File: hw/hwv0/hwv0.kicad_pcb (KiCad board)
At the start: 2 copper layers, 60.3 x 54.6 mm, 29 parts, among them J1 AVR-ISP-6, J2 PWR_IN_7-12V, J3 RS232, SW1 SW_Push, U1 ATtiny84A-MU, U2 LCD_1602, U3 MAX232I, U4 L7805

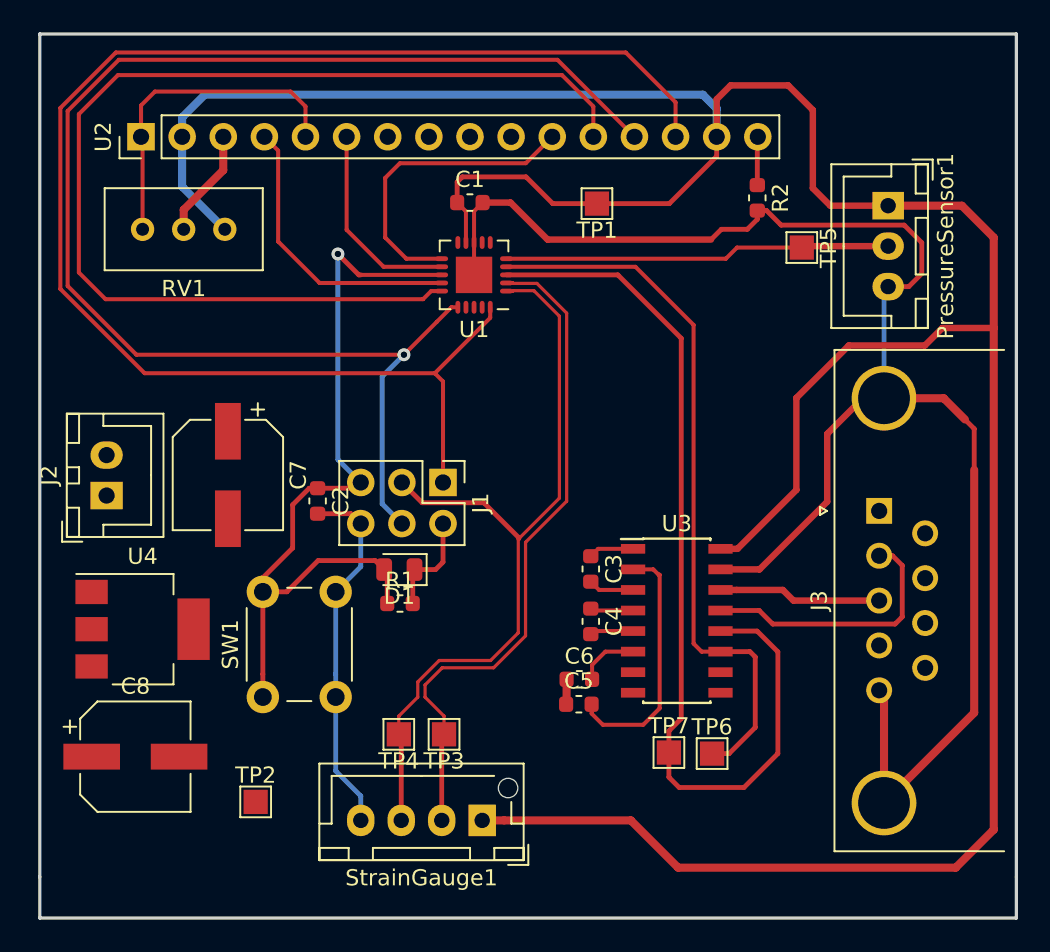
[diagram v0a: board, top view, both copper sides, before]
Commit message: finished PCB
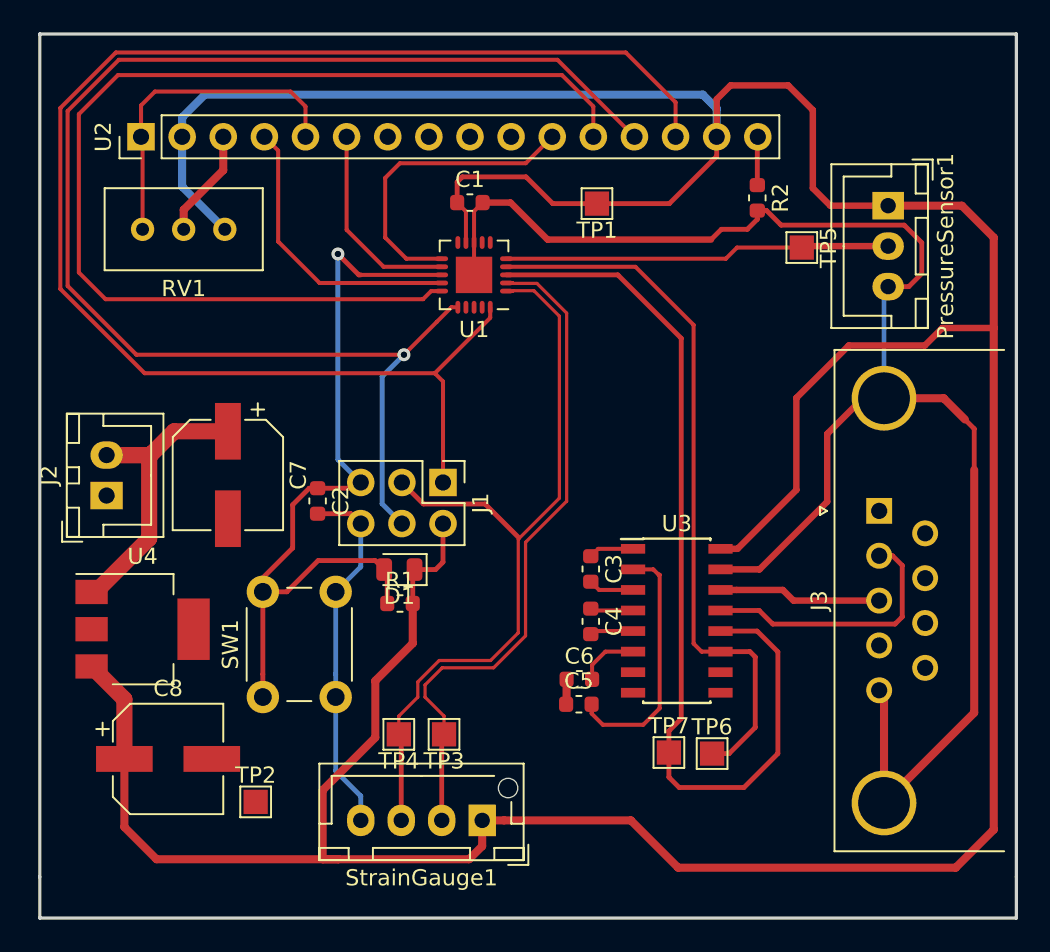
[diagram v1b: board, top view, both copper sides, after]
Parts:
- moved C8 2.02 mm to (77.8, 154.6)
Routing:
- net +5V: track 196.1 -> 250.8 mm
- net Net-(C7-Pad1): track 0.00 -> 20.8 mm
- added copper zone on B.Cu, net GNDD
- added copper zone on F.Cu, net GNDD
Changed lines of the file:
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@@
     (thickness 1.6)
     (drawings 6)
-    (tracks 260)
+    (tracks 281)
     (zones 0)
     (modules 29)
@@
   )
   (module Capacitor_SMD:CP_Elec_6.3x3 (layer F.Cu)
-    (at 75.7555 154.4955)
+    (at 77.7748 154.6352)
     (descr "SMT capacitor, aluminium electrolytic, 6.3x3, Nichicon ")
     (tags "Capacitor Electrolytic")
@@
   (segment (start 95.631 118.999) (end 95.631 120.269) (width 0.3) (layer F.Cu) (net 1))
   (segment (start 95.9485 118.6815) (end 95.631 118.999) (width 0.3) (layer F.Cu) (net 1))
+  (segment (start 97.1785 158.4325) (end 97.1785 160.0219) (width 0.5) (layer F.Cu) (net 1))
+  (segment (start 97.1785 160.0219) (end 96.3676 160.8328) (width 0.5) (layer F.Cu) (net 1))
+  (segment (start 96.3676 160.8328) (end 88.2904 160.8328) (width 0.5) (layer F.Cu) (net 1))
+  (segment (start 75.0748 150.9463) (end 73.05 148.9215) (width 1) (layer F.Cu) (net 1))
+  (segment (start 75.0748 154.6352) (end 75.0748 150.9463) (width 1) (layer F.Cu) (net 1))
+  (segment (start 88.2904 160.8328) (end 77.0636 160.8328) (width 0.5) (layer F.Cu) (net 1))
+  (segment (start 75.0748 158.844) (end 75.0748 154.6352) (width 0.5) (layer F.Cu) (net 1))
+  (segment (start 77.0636 160.8328) (end 75.0748 158.844) (width 0.5) (layer F.Cu) (net 1))
+  (segment (start 92.888 147.4976) (end 92.888 145.034) (width 0.5) (layer F.Cu) (net 1))
+  (segment (start 90.5764 149.8092) (end 92.888 147.4976) (width 0.5) (layer F.Cu) (net 1))
+  (segment (start 90.5764 153.3144) (end 90.5764 149.8092) (width 0.5) (layer F.Cu) (net 1))
+  (segment (start 87.3252 156.5656) (end 90.5764 153.3144) (width 0.5) (layer F.Cu) (net 1))
+  (segment (start 88.2904 160.8328) (end 87.3252 160.8328) (width 0.5) (layer F.Cu) (net 1))
+  (segment (start 87.3252 160.8328) (end 87.3252 156.5656) (width 0.5) (layer F.Cu) (net 1))
   (segment (start 76.2 116.300393) (end 76.10405 116.204443) (width 0.25) (layer F.Cu) (net 2))
   (segment (start 76.2 121.92) (end 76.2 116.300393) (width 0.25) (layer F.Cu) (net 2))
@@
   (segment (start 93.649451 150.064249) (end 93.649451 150.818555) (width 0.2) (layer F.Cu) (net 12))
   (segment (start 94.7082 149.0055) (end 93.649451 150.064249) (width 0.2) (layer F.Cu) (net 12))
-  (segment (start 92.1785 153.266605) (end 92.027451 153.115556) (width 0.3) (layer F.Cu) (net 24))
-  (segment (start 92.1785 158.4325) (end 92.1785 153.266605) (width 0.3) (layer F.Cu) (net 24))
-  (segment (start 92.027451 151.990555) (end 93.199451 150.818555) (width 0.2) (layer F.Cu) (net 24))
-  (segment (start 92.027451 153.115556) (end 92.027451 151.990555) (width 0.2) (layer F.Cu) (net 24))
-  (segment (start 98.675433 125.735663) (end 99.075433 125.735663) (width 0.2) (layer F.Cu) (net 24))
-  (segment (start 99.075433 125.735663) (end 99.100433 125.710663) (width 0.2) (layer F.Cu) (net 24))
-  (segment (start 99.100433 125.710663) (end 100.373463 125.710663) (width 0.2) (layer F.Cu) (net 24))
-  (segment (start 100.373463 125.710663) (end 101.9465 127.2837) (width 0.2) (layer F.Cu) (net 24))
-  (segment (start 101.9465 127.2837) (end 101.9465 138.5273) (width 0.2) (layer F.Cu) (net 24))
-  (segment (start 99.4065 141.0673) (end 99.4065 146.8458) (width 0.2) (layer F.Cu) (net 24))
-  (segment (start 99.4065 146.8458) (end 97.6968 148.5555) (width 0.2) (layer F.Cu) (net 24))
-  (segment (start 97.6968 148.5555) (end 94.5218 148.5555) (width 0.2) (layer F.Cu) (net 24))
-  (segment (start 94.5218 148.5555) (end 93.199451 149.877849) (width 0.2) (layer F.Cu) (net 24))
-  (segment (start 93.199451 149.877849) (end 93.199451 150.818555) (width 0.2) (layer F.Cu) (net 24))
   (segment (start 111.898557 146.73705) (end 114.16155 146.73705) (width 0.3) (layer F.Cu) (net 13))
   (segment (start 114.16155 146.73705) (end 115.443 148.0185) (width 0.3) (layer F.Cu) (net 13))
@@
   (segment (start 121.700556 144.855049) (end 116.407049 144.855049) (width 0.4) (layer F.Cu) (net 20))
   (segment (start 116.407049 144.855049) (end 115.74905 144.19705) (width 0.4) (layer F.Cu) (net 20))
+  (segment (start 76.6807 135.8665) (end 73.9775 135.8665) (width 1) (layer F.Cu) (net 21))
+  (segment (start 81.4705 134.3965) (end 78.1507 134.3965) (width 1) (layer F.Cu) (net 21))
+  (segment (start 78.1507 134.3965) (end 76.6807 135.8665) (width 1) (layer F.Cu) (net 21))
+  (segment (start 73.3 144.3215) (end 73.05 144.3215) (width 1) (layer F.Cu) (net 21))
+  (segment (start 76.6064 141.0151) (end 73.3 144.3215) (width 1) (layer F.Cu) (net 21))
+  (segment (start 76.6064 135.8392) (end 76.6064 141.0151) (width 1) (layer F.Cu) (net 21))
+  (segment (start 73.9775 135.8665) (end 76.5791 135.8665) (width 1) (layer F.Cu) (net 21))
+  (segment (start 76.5791 135.8665) (end 76.6064 135.8392) (width 1) (layer F.Cu) (net 21))
   (segment (start 114.20405 119.34895) (end 114.173 119.38) (width 0.4) (layer F.Cu) (net 22))
   (segment (start 114.173 116.235493) (end 114.20405 116.204443) (width 0.3) (layer F.Cu) (net 22))
@@
   (segment (start 94.757951 131.316855) (end 94.251096 130.81) (width 0.25) (layer F.Cu) (net 23))
   (segment (start 94.757951 137.558056) (end 94.757951 131.316855) (width 0.25) (layer F.Cu) (net 23))
+  (segment (start 92.1785 153.266605) (end 92.027451 153.115556) (width 0.3) (layer F.Cu) (net 24))
+  (segment (start 92.1785 158.4325) (end 92.1785 153.266605) (width 0.3) (layer F.Cu) (net 24))
+  (segment (start 92.027451 151.990555) (end 93.199451 150.818555) (width 0.2) (layer F.Cu) (net 24))
+  (segment (start 92.027451 153.115556) (end 92.027451 151.990555) (width 0.2) (layer F.Cu) (net 24))
+  (segment (start 98.675433 125.735663) (end 99.075433 125.735663) (width 0.2) (layer F.Cu) (net 24))
+  (segment (start 99.075433 125.735663) (end 99.100433 125.710663) (width 0.2) (layer F.Cu) (net 24))
+  (segment (start 99.100433 125.710663) (end 100.373463 125.710663) (width 0.2) (layer F.Cu) (net 24))
+  (segment (start 100.373463 125.710663) (end 101.9465 127.2837) (width 0.2) (layer F.Cu) (net 24))
+  (segment (start 101.9465 127.2837) (end 101.9465 138.5273) (width 0.2) (layer F.Cu) (net 24))
+  (segment (start 99.4065 141.0673) (end 99.4065 146.8458) (width 0.2) (layer F.Cu) (net 24))
+  (segment (start 99.4065 146.8458) (end 97.6968 148.5555) (width 0.2) (layer F.Cu) (net 24))
+  (segment (start 97.6968 148.5555) (end 94.5218 148.5555) (width 0.2) (layer F.Cu) (net 24))
+  (segment (start 94.5218 148.5555) (end 93.199451 149.877849) (width 0.2) (layer F.Cu) (net 24))
+  (segment (start 93.199451 149.877849) (end 93.199451 150.818555) (width 0.2) (layer F.Cu) (net 24))
   (segment (start 101.9465 138.5273) (end 99.441 141.0328) (width 0.2) (layer F.Cu) (net 24))
   (segment (start 99.441 141.0328) (end 99.4065 141.0673) (width 0.2) (layer F.Cu) (net 24))
-  (segment (start 99.441 140.97) (end 99.441 141.0328) (width 0.3) (layer F.Cu) (net 24))
-  (segment (start 97.282 138.811) (end 99.441 140.97) (width 0.3) (layer F.Cu) (net 24))
-  (segment (start 92.217951 137.558056) (end 93.470895 138.811) (width 0.3) (layer F.Cu) (net 24))
-  (segment (start 93.470895 138.811) (end 97.282 138.811) (width 0.3) (layer F.Cu) (net 24))
+  (segment (start 97.3582 138.8872) (end 99.441 140.97) (width 0.3) (layer F.Cu) (net 24))
+  (segment (start 92.217951 137.558056) (end 93.547095 138.8872) (width 0.3) (layer F.Cu) (net 24))
+  (segment (start 93.547095 138.8872) (end 97.3582 138.8872) (width 0.3) (layer F.Cu) (net 24))
   (segment (start 75.82041 129.667) (end 92.344096 129.667) (width 0.25) (layer F.Cu) (net 25))
   (segment (start 106.58405 116.204443) (end 101.827618 111.448011) (width 0.25) (layer F.Cu) (net 25))
@@
   (segment (start 92.217951 140.098056) (end 90.9955 138.875605) (width 0.3) (layer B.Cu) (net 25))
   (segment (start 90.9955 138.875605) (end 90.9955 131.015596) (width 0.3) (layer B.Cu) (net 25))
+  (zone (net 2) (net_name GNDD) (layer B.Cu) (hatch none 0.508)
+    (connect_pads (clearance 0.508))
+    (min_thickness 0.254)
+    (fill yes (arc_segments 16) (thermal_gap 0.508) (thermal_bridge_width 0.508))
+    (polygon
+      (pts
+        (xy 69.85 109.855) (xy 130.175 109.855) (xy 130.175 164.465) (xy 69.85 164.465)
+      )
+    )
+  )
+  (zone (net 2) (net_name GNDD) (layer F.Cu) (hatch none 0.508)
+    (connect_pads (clearance 0.508))
+    (min_thickness 0.254)
+    (fill yes (arc_segments 16) (thermal_gap 0.508) (thermal_bridge_width 0.508))
+    (polygon
+      (pts
+        (xy 69.85 109.855) (xy 130.175 109.855) (xy 130.175 164.465) (xy 69.85 164.465)
+      )
+    )
+  )
 )
